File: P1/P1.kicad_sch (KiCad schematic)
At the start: 68 parts, among them J1 USB_C, J2 Conn_01x04_Pin, J3 Conn_01x04_Pin, J4 Conn_01x04_Pin, J5 Conn_01x05, J6 Conn_01x05, J7 Conn_01x02_Pin, SW1 SW_SPDT, U1 STM32F103C8T6, U2 MCP2542FD, U3 AMS1117-3.3, U5 74HC164, X1 OXETDLJANF-8MHZ

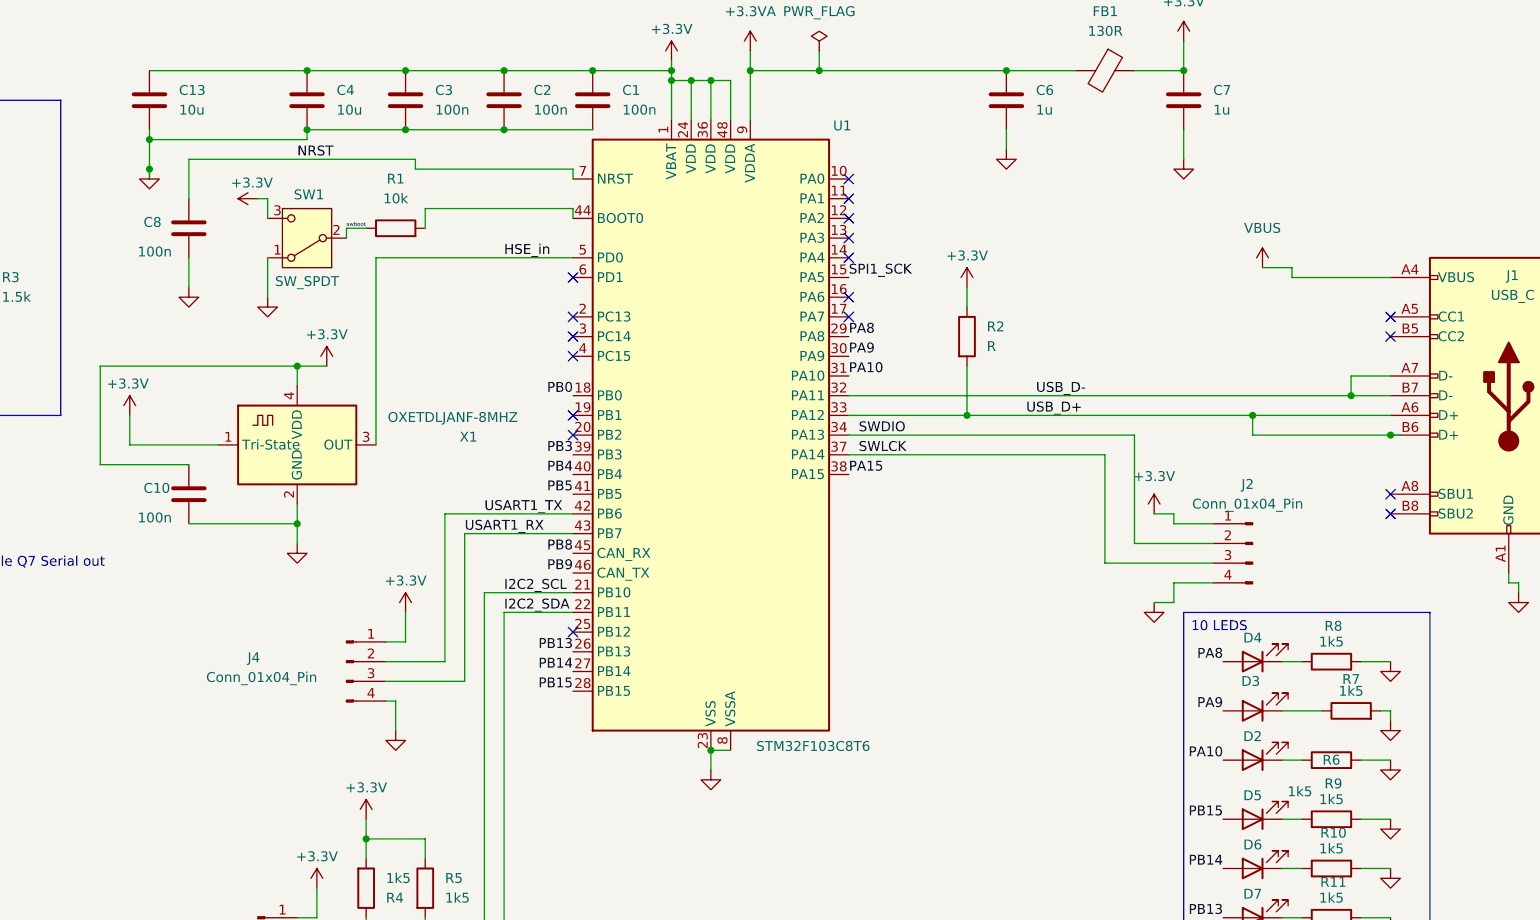
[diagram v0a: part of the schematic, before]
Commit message: Reviewed version for manufacture
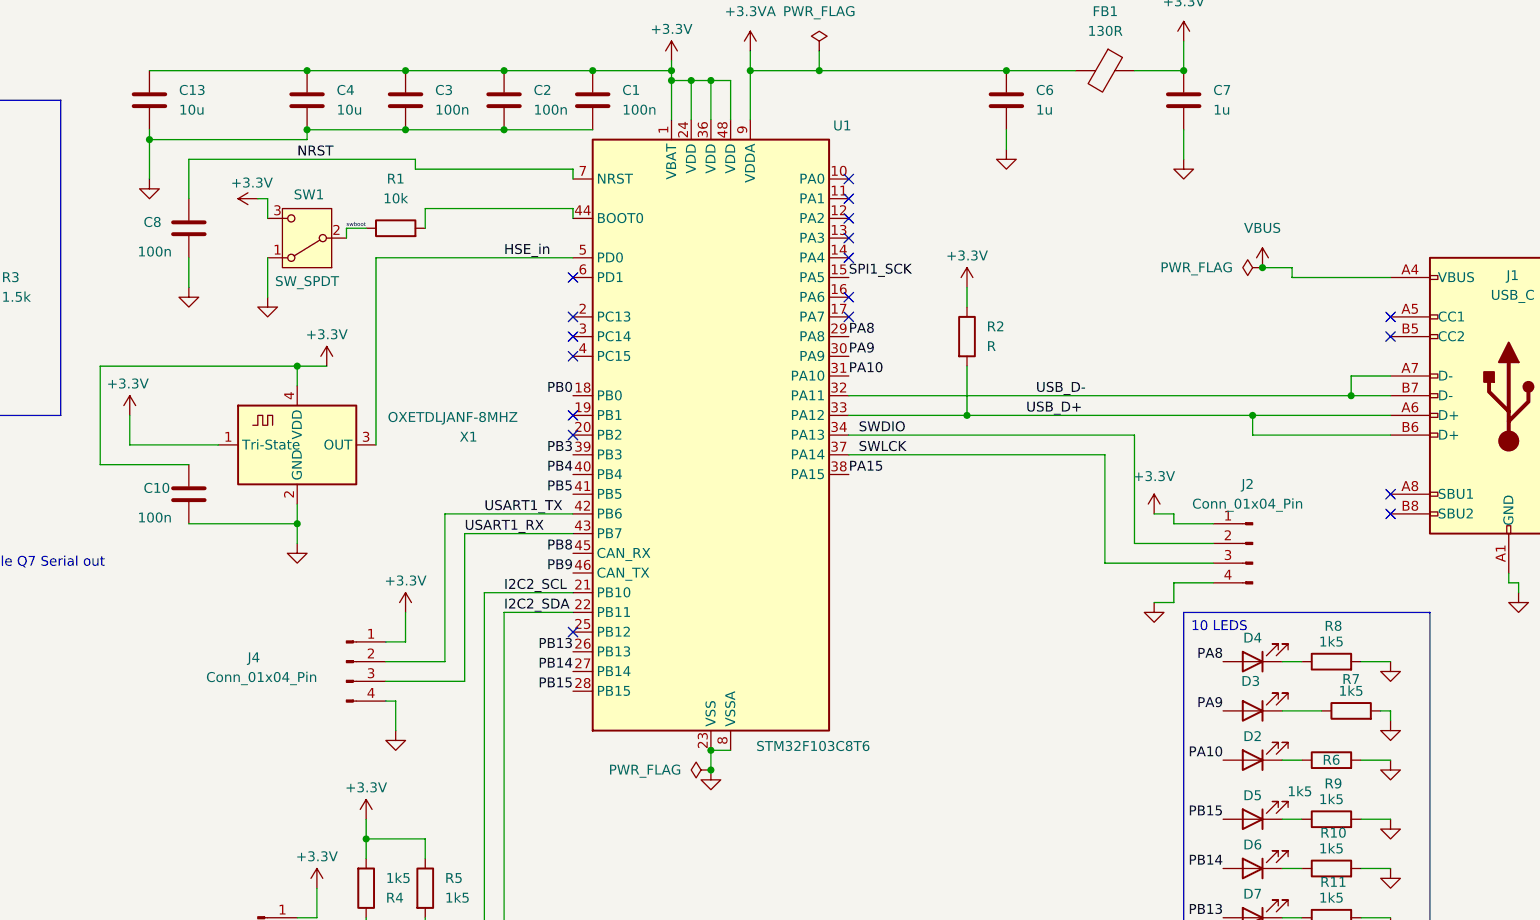
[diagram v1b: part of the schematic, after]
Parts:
- C1, C2, C3, C6: footprint Capacitor_SMD:C_0402_1005Metric -> Capacitor_SMD:C_0603_1608Metric
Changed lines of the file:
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@@
 	)
 	(junction
-		(at 279.4 77.47)
-		(diameter 0)
-		(color 0 0 0 0)
-	)
-	(junction
 		(at 191.77 118.11)
 		(diameter 0)
@@
 	)
 	(junction
-		(at 119.38 43.18)
+		(at 191.77 120.65)
 		(diameter 0)
 		(color 0 0 0 0)
@@
 	)
 	(junction
+		(at 262.89 55.88)
+		(diameter 0)
+		(color 0 0 0 0)
+	)
+	(junction
 		(at 138.43 68.58)
 		(diameter 0)
@@
 	(wire
 		(pts
-			(xy 280.67 77.47) (xy 279.4 77.47)
-		)
-		(stroke
-			(width 0)
-			(type default)
-		)
-	)
-	(wire
-		(pts
 			(xy 33.02 156.21) (xy 29.21 156.21)
 		)
@@
 	(wire
 		(pts
-			(xy 119.38 39.37) (xy 119.38 43.18)
+			(xy 119.38 39.37) (xy 119.38 44.45)
+		)
+		(stroke
+			(width 0)
+			(type default)
+		)
+	)
+	(wire
+		(pts
+			(xy 261.62 77.47) (xy 279.4 77.47)
 		)
 		(stroke
@@
 	(wire
 		(pts
-			(xy 119.38 43.18) (xy 119.38 44.45)
-		)
-		(stroke
-			(width 0)
-			(type default)
-		)
-	)
-	(wire
-		(pts
 			(xy 246.38 91.44) (xy 256.54 91.44)
 		)
@@
 	(wire
 		(pts
-			(xy 279.4 77.47) (xy 261.62 77.47)
-		)
-		(stroke
-			(width 0)
-			(type default)
-		)
-	)
-	(wire
-		(pts
 			(xy 205.74 30.48) (xy 196.85 30.48)
 		)
@@
 			)
 		)
-		(property "Footprint" "Capacitor_SMD:C_0402_1005Metric"
+		(property "Footprint" "Capacitor_SMD:C_0603_1608Metric"
 			(at 177.4952 38.1 0)
 			(effects
@@
 	(symbol
 		(lib_id "power:GND")
-		(at 119.38 43.18 0)
+		(at 119.38 44.45 0)
 		(unit 1)
 		(exclude_from_sim no)
@@
 		(fields_autoplaced yes)
 		(property "Reference" "#PWR03"
-			(at 119.38 49.53 0)
+			(at 119.38 50.8 0)
 			(effects
 				(font
@@
 		)
 		(property "Value" "GND"
-			(at 119.38 48.26 0)
+			(at 119.38 49.53 0)
 			(effects
 				(font
@@
 		)
 		(property "Footprint" ""
-			(at 119.38 43.18 0)
+			(at 119.38 44.45 0)
 			(effects
 				(font
@@
 		)
 		(property "Datasheet" ""
-			(at 119.38 43.18 0)
+			(at 119.38 44.45 0)
 			(effects
 				(font
@@
 		)
 		(property "Description" "Power symbol creates a global label with name \"GND\" , ground"
-			(at 119.38 43.18 0)
+			(at 119.38 44.45 0)
 			(effects
 				(font
@@
 	)
 	(symbol
+		(lib_id "power:PWR_FLAG")
+		(at 262.89 55.88 90)
+		(unit 1)
+		(exclude_from_sim no)
+		(in_bom yes)
+		(on_board yes)
+		(dnp no)
+		(fields_autoplaced yes)
+		(property "Reference" "#FLG03"
+			(at 260.985 55.88 0)
+			(effects
+				(font
+					(size 1.27 1.27)
+				)
+				(hide yes)
+			)
+		)
+		(property "Value" "PWR_FLAG"
+			(at 259.08 55.8799 90)
+			(effects
+				(font
+					(size 1.27 1.27)
+				)
+				(justify left)
+			)
+		)
+		(property "Footprint" ""
+			(at 262.89 55.88 0)
+			(effects
+				(font
+					(size 1.27 1.27)
+				)
+				(hide yes)
+			)
+		)
+		(property "Datasheet" "~"
+			(at 262.89 55.88 0)
+			(effects
+				(font
+					(size 1.27 1.27)
+				)
+				(hide yes)
+			)
+		)
+		(property "Description" "Special symbol for telling ERC where power comes from"
+			(at 262.89 55.88 0)
+			(effects
+				(font
+					(size 1.27 1.27)
+				)
+				(hide yes)
+			)
+		)
+		(pin "1"
+		)
+		(instances
+			(project ""
+				(path "/71953e7d-f25f-4698-84c8-ace8e153d13d"
+					(reference "#FLG03")
+					(unit 1)
+				)
+			)
+		)
+	)
+	(symbol
 		(lib_id "Device:FerriteBead")
 		(at 242.57 30.48 270)
@@
 	)
 	(symbol
+		(lib_id "power:PWR_FLAG")
+		(at 191.77 120.65 90)
+		(unit 1)
+		(exclude_from_sim no)
+		(in_bom yes)
+		(on_board yes)
+		(dnp no)
+		(fields_autoplaced yes)
+		(property "Reference" "#FLG02"
+			(at 189.865 120.65 0)
+			(effects
+				(font
+					(size 1.27 1.27)
+				)
+				(hide yes)
+			)
+		)
+		(property "Value" "PWR_FLAG"
+			(at 187.96 120.6499 90)
+			(effects
+				(font
+					(size 1.27 1.27)
+				)
+				(justify left)
+			)
+		)
+		(property "Footprint" ""
+			(at 191.77 120.65 0)
+			(effects
+				(font
+					(size 1.27 1.27)
+				)
+				(hide yes)
+			)
+		)
+		(property "Datasheet" "~"
+			(at 191.77 120.65 0)
+			(effects
+				(font
+					(size 1.27 1.27)
+				)
+				(hide yes)
+			)
+		)
+		(property "Description" "Special symbol for telling ERC where power comes from"
+			(at 191.77 120.65 0)
+			(effects
+				(font
+					(size 1.27 1.27)
+				)
+				(hide yes)
+			)
+		)
+		(pin "1"
+		)
+		(instances
+			(project ""
+				(path "/71953e7d-f25f-4698-84c8-ace8e153d13d"
+					(reference "#FLG02")
+					(unit 1)
+				)
+			)
+		)
+	)
+	(symbol
 		(lib_id "power:GND")
 		(at 15.24 88.9 0)
@@
 			)
 		)
-		(property "Footprint" "Capacitor_SMD:C_0402_1005Metric"
+		(property "Footprint" "Capacitor_SMD:C_0603_1608Metric"
 			(at 166.0652 38.1 0)
 			(effects
@@
 			)
 		)
-		(property "Footprint" "Capacitor_SMD:C_0402_1005Metric"
+		(property "Footprint" "Capacitor_SMD:C_0603_1608Metric"
 			(at 230.8352 38.1 0)
 			(effects
@@
 			)
 		)
-		(property "Footprint" "Capacitor_SMD:C_0402_1005Metric"
+		(property "Footprint" "Capacitor_SMD:C_0603_1608Metric"
 			(at 153.3652 38.1 0)
 			(effects
